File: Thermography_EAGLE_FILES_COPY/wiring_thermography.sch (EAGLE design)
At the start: 19 parts

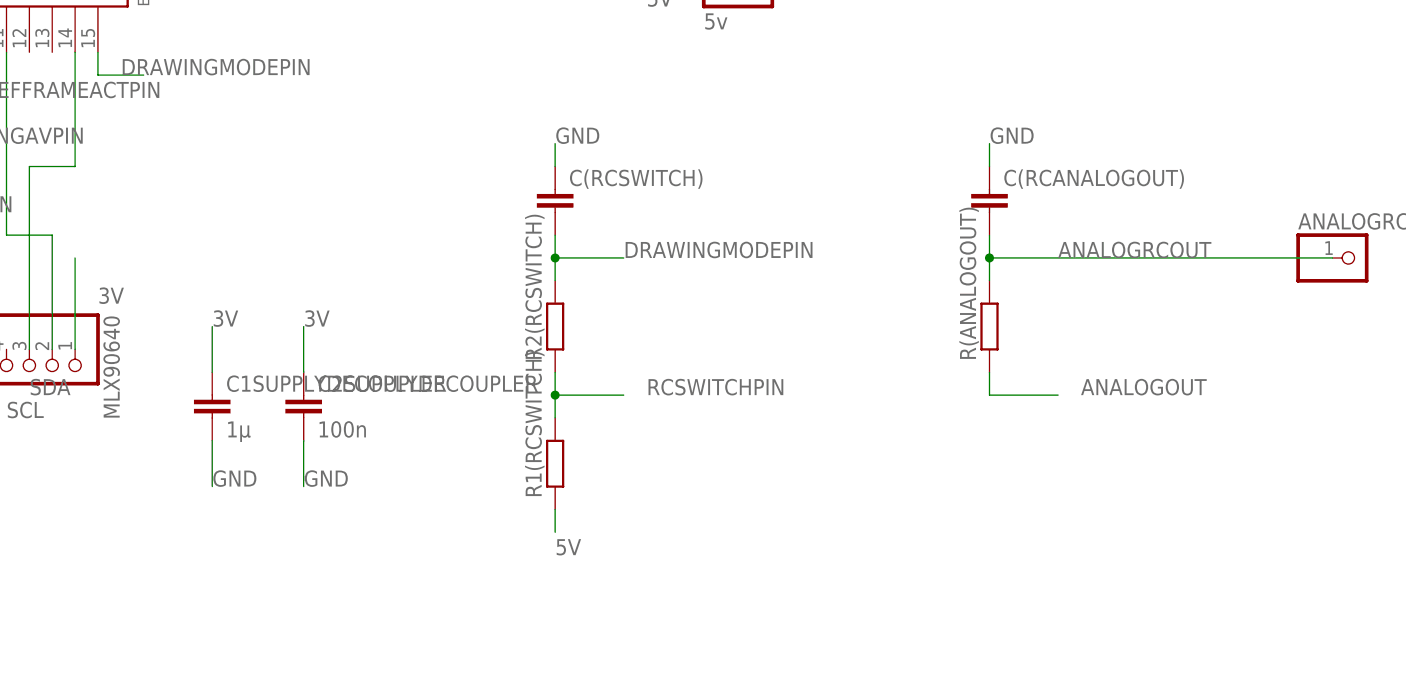
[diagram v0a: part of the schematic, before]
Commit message: updated eagle files
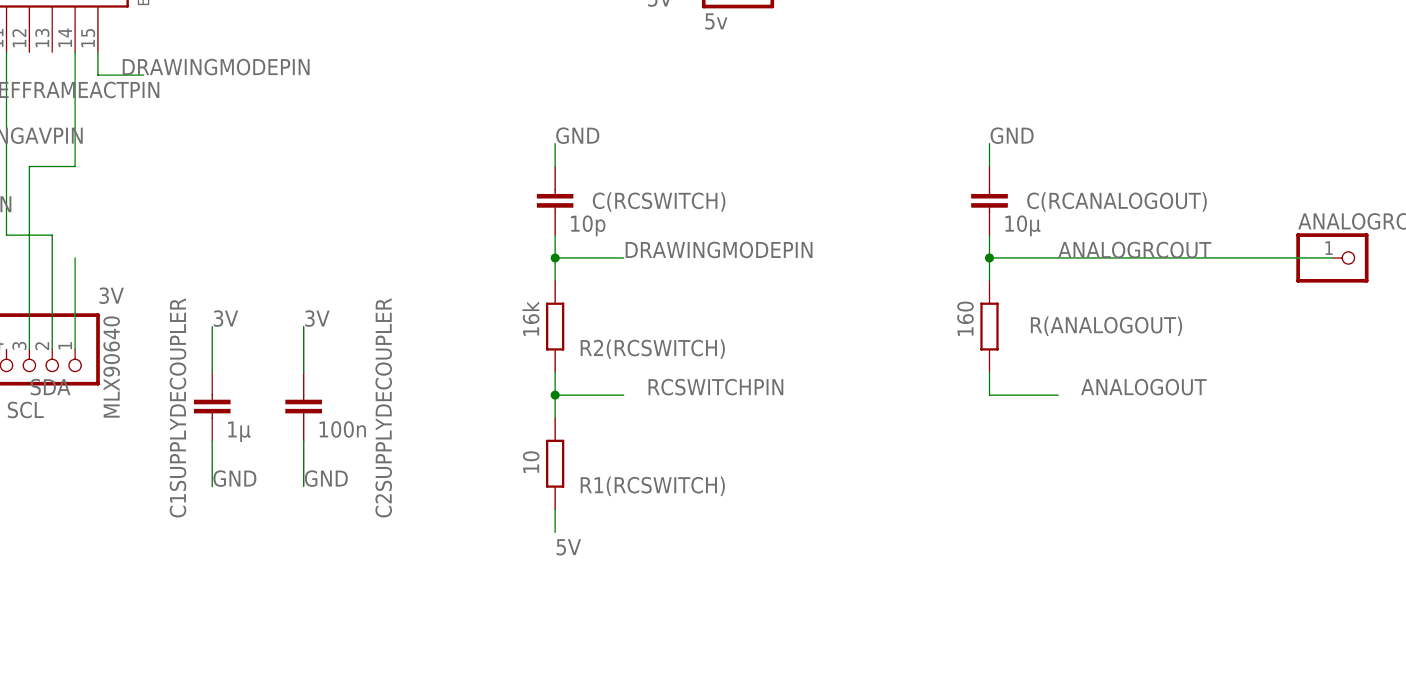
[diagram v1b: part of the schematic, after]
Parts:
- C(RCANALOGOUT): value (none) -> 10µ
- C(RCSWITCH): value (none) -> 10p
- R(ANALOGOUT): value (none) -> 160
- R1(RCSWITCH): value (none) -> 10
- R2(RCSWITCH): value (none) -> 16k
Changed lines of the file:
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@@
 <part name="C2SUPPLYDECOUPLER" library="capacitor-wima" library_urn="urn:adsk.eagle:library:116" deviceset="C" device="5/5" package3d_urn="urn:adsk.eagle:package:5428/1" value="100n"/>
 <part name="C1SUPPLYDECOUPLER" library="capacitor-wima" library_urn="urn:adsk.eagle:library:116" deviceset="C" device="5/5" package3d_urn="urn:adsk.eagle:package:5428/1" value="1µ"/>
-<part name="C(RCSWITCH)" library="capacitor-wima" library_urn="urn:adsk.eagle:library:116" deviceset="C" device="5/5" package3d_urn="urn:adsk.eagle:package:5428/1"/>
+<part name="C(RCSWITCH)" library="capacitor-wima" library_urn="urn:adsk.eagle:library:116" deviceset="C" device="5/5" package3d_urn="urn:adsk.eagle:package:5428/1" value="10p"/>
 <part name="DRAWINGMODEPIN" library="con-garry" library_urn="urn:adsk.eagle:library:147" deviceset="332-02" device="" package3d_urn="urn:adsk.eagle:package:6810/1"/>
 <part name="ROLLINGAVPIN" library="con-garry" library_urn="urn:adsk.eagle:library:147" deviceset="332-02" device="" package3d_urn="urn:adsk.eagle:package:6810/1"/>
 <part name="REFFRAMEACTPIN" library="con-garry" library_urn="urn:adsk.eagle:library:147" deviceset="332-02" device="" package3d_urn="urn:adsk.eagle:package:6810/1"/>
 <part name="REFTAKEPIN" library="con-garry" library_urn="urn:adsk.eagle:library:147" deviceset="332-02" device="" package3d_urn="urn:adsk.eagle:package:6810/1"/>
-<part name="C(RCANALOGOUT)" library="capacitor-wima" library_urn="urn:adsk.eagle:library:116" deviceset="C" device="5/5" package3d_urn="urn:adsk.eagle:package:5428/1"/>
+<part name="C(RCANALOGOUT)" library="capacitor-wima" library_urn="urn:adsk.eagle:library:116" deviceset="C" device="5/5" package3d_urn="urn:adsk.eagle:package:5428/1" value="10µ"/>
 <part name="ANALOGRCOUTPIN" library="pinhead" library_urn="urn:adsk.eagle:library:325" deviceset="PINHD-1X1" device="" package3d_urn="urn:adsk.eagle:package:22485/2"/>
 <part name="GNDPIN" library="pinhead" library_urn="urn:adsk.eagle:library:325" deviceset="PINHD-1X1" device="" package3d_urn="urn:adsk.eagle:package:22485/2" value="gnd"/>
@@
 <part name="GNDPIN3" library="pinhead" library_urn="urn:adsk.eagle:library:325" deviceset="PINHD-1X1" device="" package3d_urn="urn:adsk.eagle:package:22485/2" value="gnd"/>
 <part name="5VPIN" library="pinhead" library_urn="urn:adsk.eagle:library:325" deviceset="PINHD-1X1" device="" package3d_urn="urn:adsk.eagle:package:22485/2" value="5v"/>
-<part name="FRAME1" library="frames" library_urn="urn:adsk.eagle:library:229" deviceset="DINA4_L" device="" value="azazaz"/>
 <part name="GND1" library="supply1" library_urn="urn:adsk.eagle:library:371" deviceset="GND" device=""/>
 <part name="LCDSPI" library="pinhead" library_urn="urn:adsk.eagle:library:325" deviceset="PINHD-1X10" device="" package3d_urn="urn:adsk.eagle:package:22406/2"/>
-<part name="R1(RCSWITCH)" library="rcl" library_urn="urn:adsk.eagle:library:334" deviceset="R-EU_" device="0207/7" package3d_urn="urn:adsk.eagle:package:23493/2"/>
-<part name="R2(RCSWITCH)" library="rcl" library_urn="urn:adsk.eagle:library:334" deviceset="R-EU_" device="0207/7" package3d_urn="urn:adsk.eagle:package:23493/2"/>
-<part name="R(ANALOGOUT)" library="rcl" library_urn="urn:adsk.eagle:library:334" deviceset="R-EU_" device="0207/7" package3d_urn="urn:adsk.eagle:package:23493/2"/>
+<part name="R1(RCSWITCH)" library="rcl" library_urn="urn:adsk.eagle:library:334" deviceset="R-EU_" device="0207/7" package3d_urn="urn:adsk.eagle:package:23493/2" value="10"/>
+<part name="R2(RCSWITCH)" library="rcl" library_urn="urn:adsk.eagle:library:334" deviceset="R-EU_" device="0207/7" package3d_urn="urn:adsk.eagle:package:23493/2" value="16k"/>
+<part name="R(ANALOGOUT)" library="rcl" library_urn="urn:adsk.eagle:library:334" deviceset="R-EU_" device="0207/7" package3d_urn="urn:adsk.eagle:package:23493/2" value="160"/>
 </parts>
 <sheets>
@@
 </instance>
 <instance part="C2SUPPLYDECOUPLER" gate="G$1" x="93.98" y="7.62" smashed="yes">
-<attribute name="NAME" x="95.504" y="8.001" size="1.778" layer="95"/>
+<attribute name="NAME" x="103.759" y="-6.096" size="1.778" layer="95" rot="R90"/>
 <attribute name="VALUE" x="95.504" y="2.921" size="1.778" layer="96"/>
 </instance>
 <instance part="C1SUPPLYDECOUPLER" gate="G$1" x="83.82" y="7.62" smashed="yes">
-<attribute name="NAME" x="85.344" y="8.001" size="1.778" layer="95"/>
+<attribute name="NAME" x="80.899" y="-6.096" size="1.778" layer="95" rot="R90"/>
 <attribute name="VALUE" x="85.344" y="2.921" size="1.778" layer="96"/>
 </instance>
 <instance part="C(RCSWITCH)" gate="G$1" x="121.92" y="30.48" smashed="yes">
-<attribute name="NAME" x="123.444" y="30.861" size="1.778" layer="95"/>
+<attribute name="NAME" x="125.984" y="28.321" size="1.778" layer="95"/>
 <attribute name="VALUE" x="123.444" y="25.781" size="1.778" layer="96"/>
 </instance>
@@
 </instance>
 <instance part="C(RCANALOGOUT)" gate="G$1" x="170.18" y="30.48" smashed="yes">
-<attribute name="NAME" x="171.704" y="30.861" size="1.778" layer="95"/>
+<attribute name="NAME" x="174.244" y="28.321" size="1.778" layer="95"/>
 <attribute name="VALUE" x="171.704" y="25.781" size="1.778" layer="96"/>
 </instance>
@@
 <attribute name="VALUE" x="138.43" y="48.26" size="1.778" layer="96"/>
 </instance>
-<instance part="FRAME1" gate="G$1" x="-40.64" y="-58.42" smashed="yes"/>
-<instance part="FRAME1" gate="G$2" x="121.92" y="-58.42" smashed="yes">
-<attribute name="LAST_DATE_TIME" x="134.62" y="-57.15" size="2.54" layer="94"/>
-<attribute name="SHEET" x="208.28" y="-57.15" size="2.54" layer="94"/>
-<attribute name="DRAWING_NAME" x="139.7" y="-39.37" size="2.54" layer="94"/>
-</instance>
 <instance part="GND1" gate="1" x="38.1" y="-20.32" smashed="yes">
 <attribute name="VALUE" x="35.56" y="-22.86" size="1.778" layer="96"/>
@@
 </instance>
 <instance part="R1(RCSWITCH)" gate="G$1" x="121.92" y="0" smashed="yes" rot="R90">
-<attribute name="NAME" x="120.4214" y="-3.81" size="1.778" layer="95" rot="R90"/>
-<attribute name="VALUE" x="125.222" y="-3.81" size="1.778" layer="96" rot="R90"/>
+<attribute name="NAME" x="140.97" y="-1.4986" size="1.778" layer="95" rot="R180"/>
+<attribute name="VALUE" x="120.142" y="-1.27" size="1.778" layer="96" rot="R90"/>
 </instance>
 <instance part="R2(RCSWITCH)" gate="G$1" x="121.92" y="15.24" smashed="yes" rot="R90">
-<attribute name="NAME" x="120.4214" y="11.43" size="1.778" layer="95" rot="R90"/>
-<attribute name="VALUE" x="125.222" y="11.43" size="1.778" layer="96" rot="R90"/>
+<attribute name="NAME" x="140.97" y="13.7414" size="1.778" layer="95" rot="R180"/>
+<attribute name="VALUE" x="120.142" y="13.97" size="1.778" layer="96" rot="R90"/>
 </instance>
 <instance part="R(ANALOGOUT)" gate="G$1" x="170.18" y="15.24" smashed="yes" rot="R90">
-<attribute name="NAME" x="168.6814" y="11.43" size="1.778" layer="95" rot="R90"/>
-<attribute name="VALUE" x="173.482" y="11.43" size="1.778" layer="96" rot="R90"/>
+<attribute name="NAME" x="191.77" y="16.2814" size="1.778" layer="95" rot="R180"/>
+<attribute name="VALUE" x="168.402" y="13.97" size="1.778" layer="96" rot="R90"/>
 </instance>
 </instances>
